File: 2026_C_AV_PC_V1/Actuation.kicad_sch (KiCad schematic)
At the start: 55 parts, among them IC2 FAN3227TMX, IC3 FAN3227TMX, IC5 FAN3227TMX, IC8 LTC3878EGN#PBF, J12 Me-b, J13 MO-bc, J14 IGNITER, J20 Me-b, J21 MO-bc, J26 Ball_valve, Q2 STS5DNF60L, Q3 BSC093N04LSGATMA1, Q4 STS5DNF60L, Q5 BSC093N04LSGATMA1

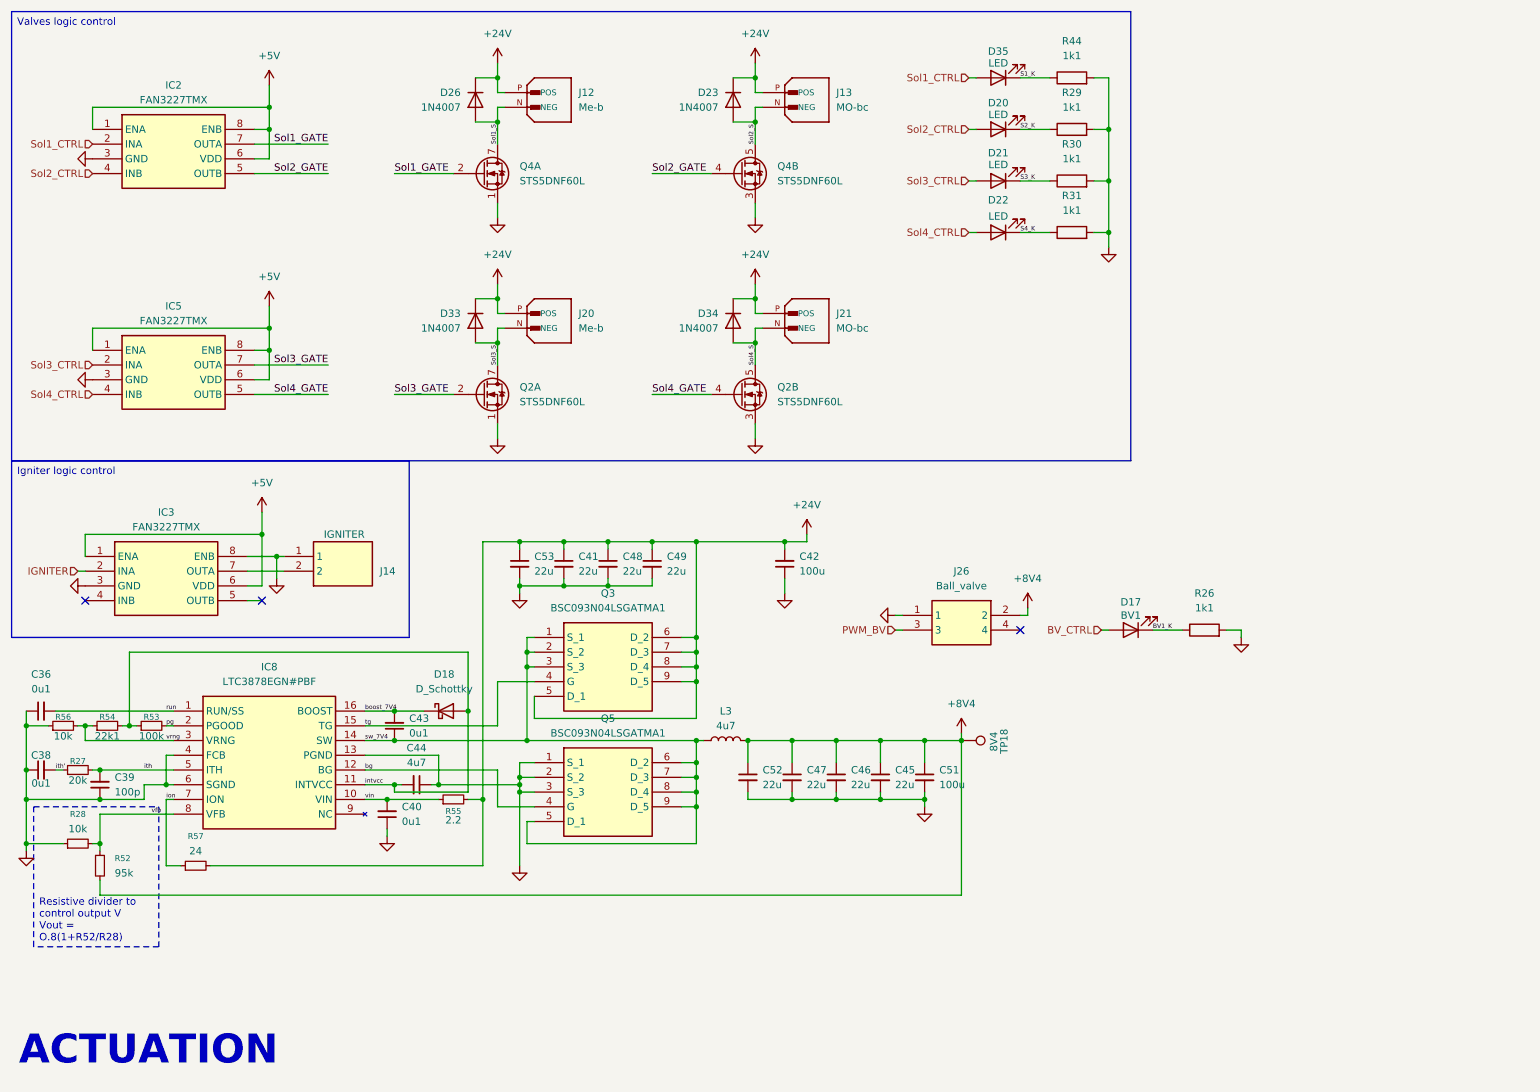
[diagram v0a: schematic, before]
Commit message: spine almost finished
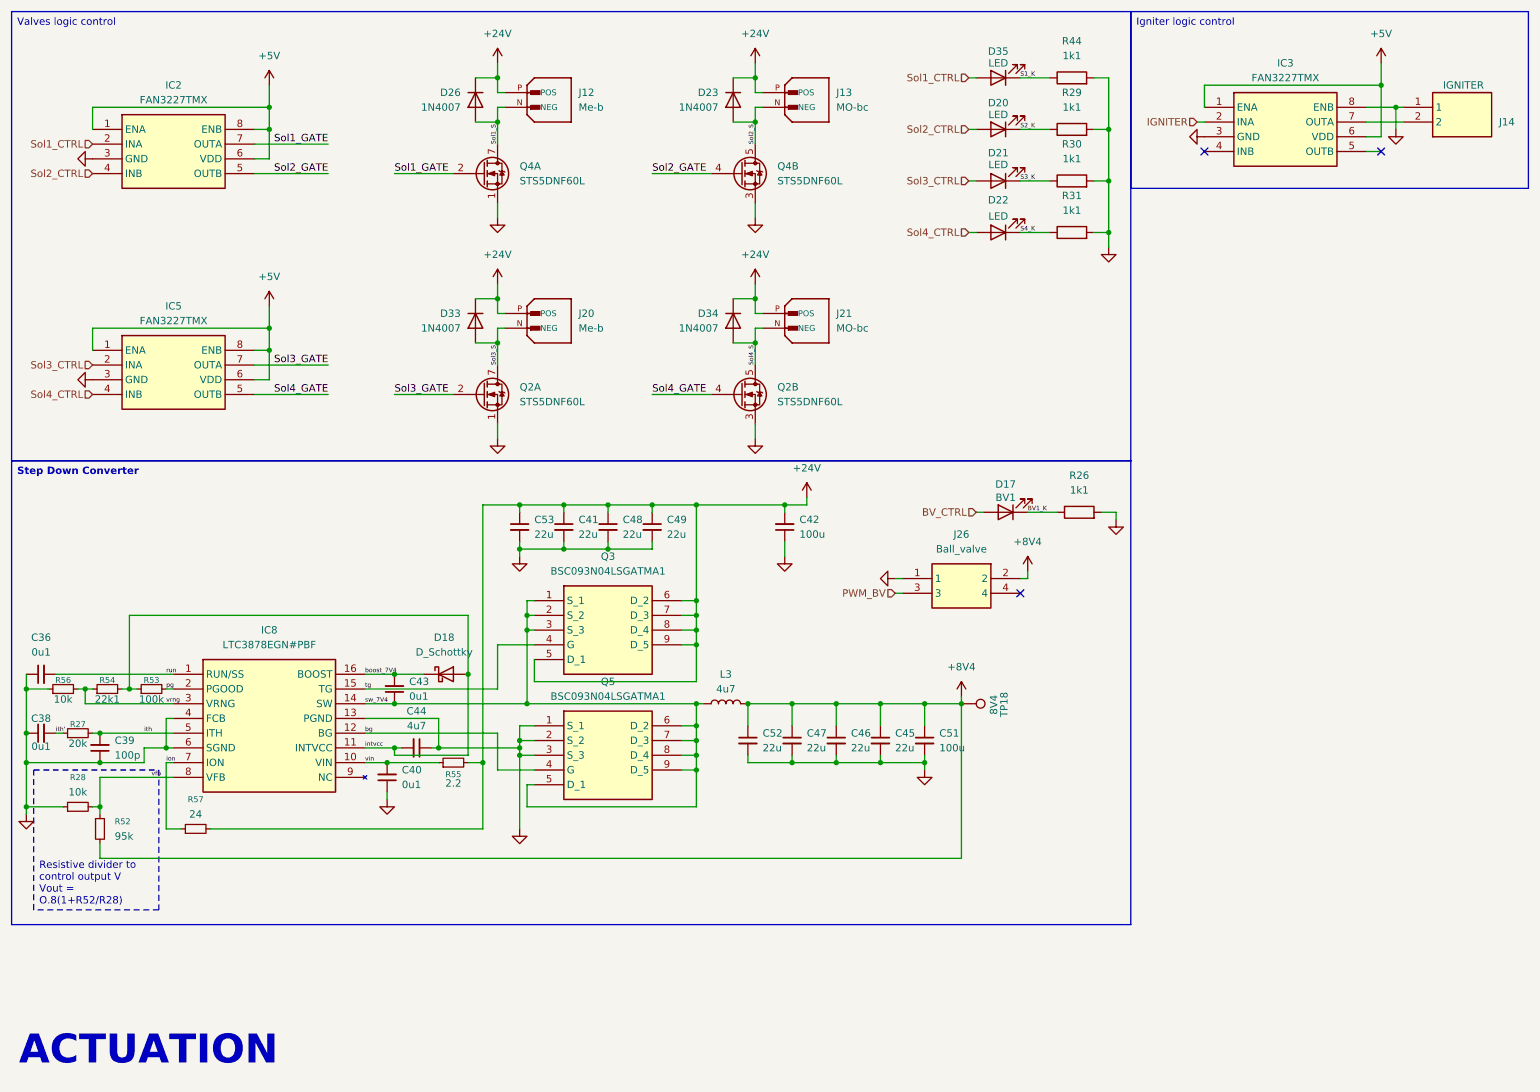
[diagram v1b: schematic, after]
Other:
- moved on the sheet: C36, C38, C39, C40, C41, C42, C43, C44, C45, C46, C47, C48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
